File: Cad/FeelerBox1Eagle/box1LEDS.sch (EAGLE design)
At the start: 13 parts

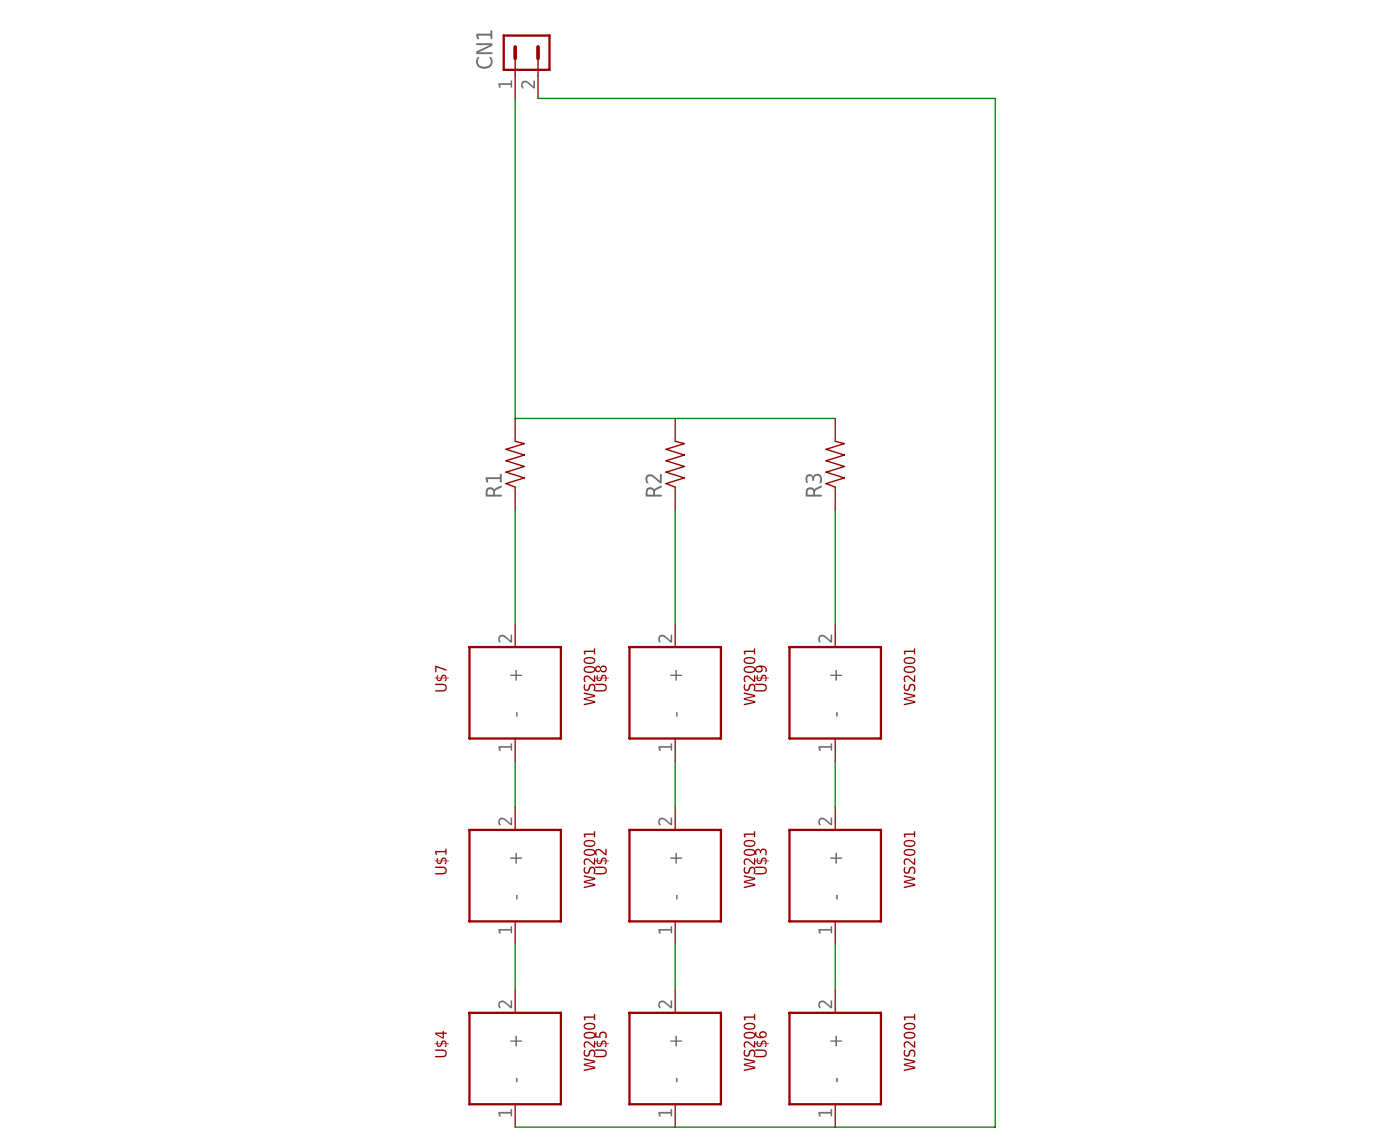
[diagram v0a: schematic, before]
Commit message: updates
bah
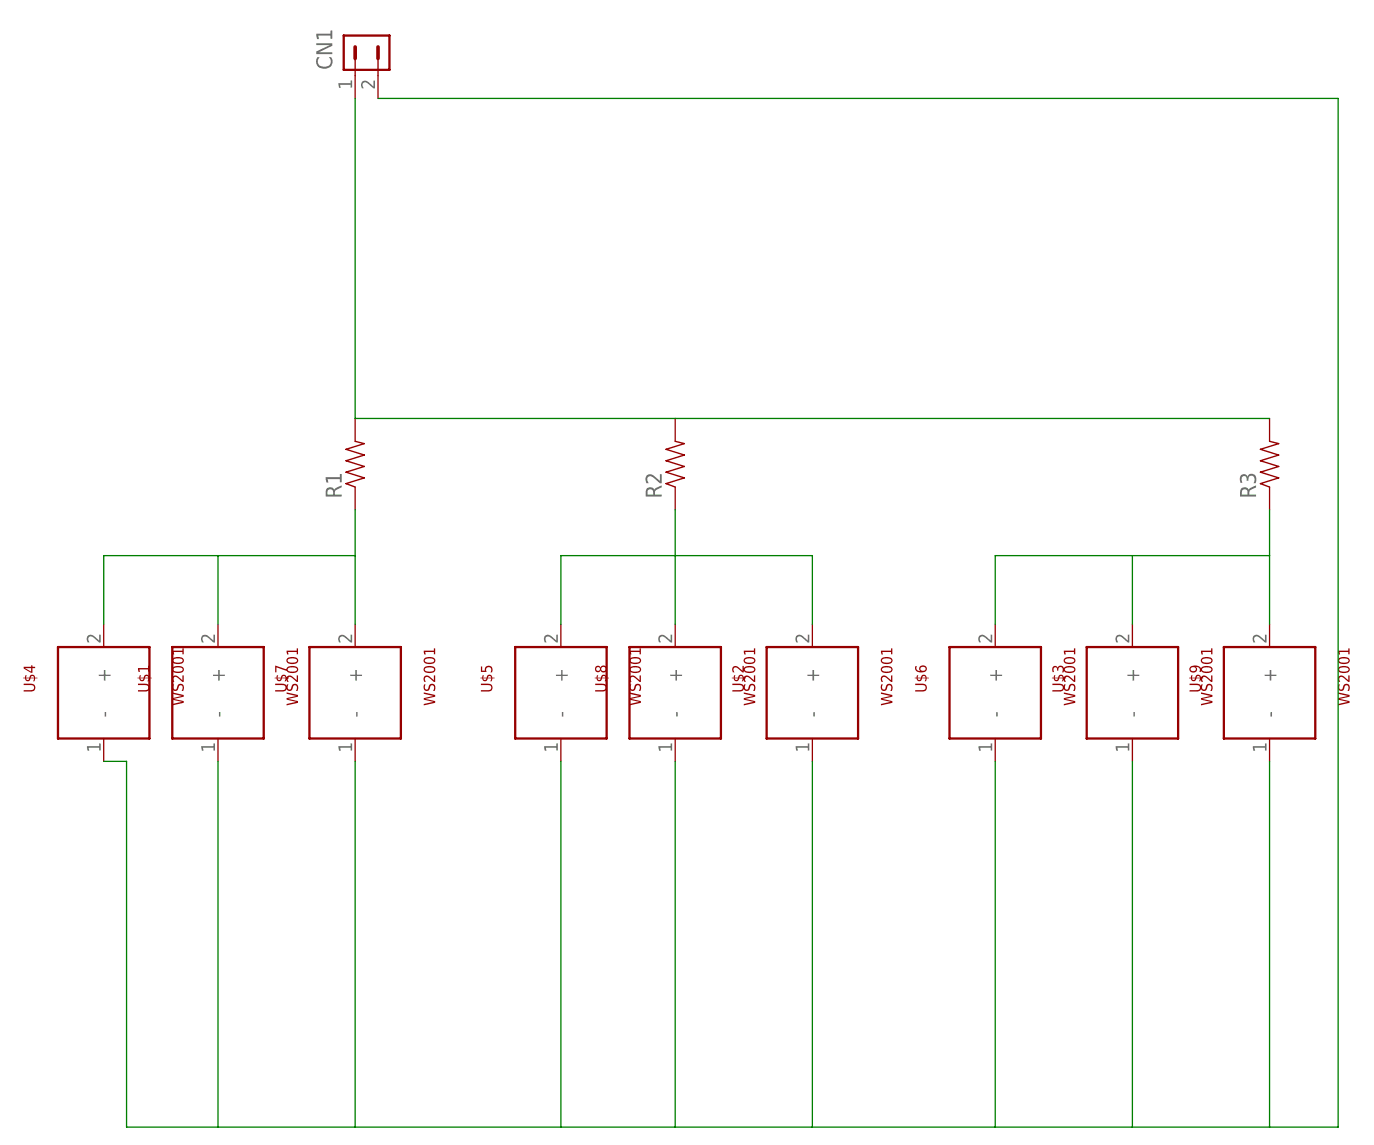
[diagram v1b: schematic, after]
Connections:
- removed net N$20: U$1.+, U$7.-
- removed net N$21: U$2.+, U$8.-
- removed net N$22: U$3.+, U$9.-
- removed net N$23: U$3.-, U$6.+
- removed net N$24: U$2.-, U$5.+
- removed net N$25: U$1.-, U$4.+
- removed net N$4: CN1.2, U$4.-, U$5.-, U$6.-
- new net GND: CN1.2, U$1.-, U$2.-, U$3.-, U$4.-, U$5.-, U$6.-, U$7.-, U$8.-, U$9.-
- net N$1: now also U$3.+, U$6.+
- net N$2: now also U$2.+, U$5.+
- net N$3: now also U$1.+, U$4.+
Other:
- moved on the sheet: CN1, R1, R3, U$1, U$2, U$3, U$4, U$5, U$6, U$7, U$9
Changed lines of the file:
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@@
 </plain>
 <instances>
-<instance part="U$1" gate="G$1" x="-2.54" y="48.26"/>
-<instance part="U$2" gate="G$1" x="15.24" y="48.26"/>
-<instance part="U$3" gate="G$1" x="33.02" y="48.26"/>
-<instance part="U$4" gate="G$1" x="-2.54" y="27.94"/>
-<instance part="U$5" gate="G$1" x="15.24" y="27.94"/>
-<instance part="U$6" gate="G$1" x="33.02" y="27.94"/>
-<instance part="U$7" gate="G$1" x="-2.54" y="68.58"/>
+<instance part="U$1" gate="G$1" x="-35.56" y="68.58"/>
+<instance part="U$2" gate="G$1" x="30.48" y="68.58"/>
+<instance part="U$3" gate="G$1" x="66.04" y="68.58"/>
+<instance part="U$4" gate="G$1" x="-48.26" y="68.58"/>
+<instance part="U$5" gate="G$1" x="2.54" y="68.58"/>
+<instance part="U$6" gate="G$1" x="50.8" y="68.58"/>
+<instance part="U$7" gate="G$1" x="-20.32" y="68.58"/>
 <instance part="U$8" gate="G$1" x="15.24" y="68.58"/>
-<instance part="U$9" gate="G$1" x="33.02" y="68.58"/>
-<instance part="R1" gate="G$1" x="-2.54" y="93.98" rot="R90"/>
+<instance part="U$9" gate="G$1" x="81.28" y="68.58"/>
+<instance part="R1" gate="G$1" x="-20.32" y="93.98" rot="R90"/>
 <instance part="R2" gate="G$1" x="15.24" y="93.98" rot="R90"/>
-<instance part="R3" gate="G$1" x="33.02" y="93.98" rot="R90"/>
-<instance part="CN1" gate="G$1" x="-2.54" y="139.7" rot="R90"/>
+<instance part="R3" gate="G$1" x="81.28" y="93.98" rot="R90"/>
+<instance part="CN1" gate="G$1" x="-20.32" y="139.7" rot="R90"/>
 </instances>
 <busses>
 </busses>
 <nets>
-<net name="N$20" class="0">
-<segment>
-<pinref part="U$1" gate="G$1" pin="+"/>
-<pinref part="U$7" gate="G$1" pin="-"/>
-<wire x1="-2.54" y1="55.88" x2="-2.54" y2="60.96" width="0.1524" layer="91"/>
-</segment>
-</net>
-<net name="N$21" class="0">
-<segment>
-<pinref part="U$2" gate="G$1" pin="+"/>
-<pinref part="U$8" gate="G$1" pin="-"/>
-<wire x1="15.24" y1="55.88" x2="15.24" y2="60.96" width="0.1524" layer="91"/>
-</segment>
-</net>
-<net name="N$22" class="0">
-<segment>
-<pinref part="U$3" gate="G$1" pin="+"/>
-<pinref part="U$9" gate="G$1" pin="-"/>
-<wire x1="33.02" y1="55.88" x2="33.02" y2="60.96" width="0.1524" layer="91"/>
-</segment>
-</net>
-<net name="N$23" class="0">
-<segment>
-<pinref part="U$6" gate="G$1" pin="+"/>
-<pinref part="U$3" gate="G$1" pin="-"/>
-<wire x1="33.02" y1="35.56" x2="33.02" y2="40.64" width="0.1524" layer="91"/>
-</segment>
-</net>
-<net name="N$24" class="0">
-<segment>
-<pinref part="U$5" gate="G$1" pin="+"/>
-<pinref part="U$2" gate="G$1" pin="-"/>
-<wire x1="15.24" y1="35.56" x2="15.24" y2="40.64" width="0.1524" layer="91"/>
-</segment>
-</net>
-<net name="N$25" class="0">
-<segment>
-<pinref part="U$4" gate="G$1" pin="+"/>
-<pinref part="U$1" gate="G$1" pin="-"/>
-<wire x1="-2.54" y1="35.56" x2="-2.54" y2="40.64" width="0.1524" layer="91"/>
-</segment>
-</net>
 <net name="N$1" class="0">
 <segment>
 <pinref part="U$9" gate="G$1" pin="+"/>
 <pinref part="R3" gate="G$1" pin="1"/>
-<wire x1="33.02" y1="76.2" x2="33.02" y2="88.9" width="0.1524" layer="91"/>
+<wire x1="81.28" y1="76.2" x2="81.28" y2="83.82" width="0.1524" layer="91"/>
+<pinref part="U$6" gate="G$1" pin="+"/>
+<wire x1="50.8" y1="76.2" x2="50.8" y2="83.82" width="0.1524" layer="91"/>
+<wire x1="50.8" y1="83.82" x2="66.04" y2="83.82" width="0.1524" layer="91"/>
+<wire x1="66.04" y1="83.82" x2="81.28" y2="83.82" width="0.1524" layer="91"/>
+<wire x1="81.28" y1="83.82" x2="81.28" y2="88.9" width="0.1524" layer="91"/>
+<pinref part="U$3" gate="G$1" pin="+"/>
+<wire x1="66.04" y1="76.2" x2="66.04" y2="83.82" width="0.1524" layer="91"/>
 </segment>
 </net>
@@
 <pinref part="U$8" gate="G$1" pin="+"/>
 <pinref part="R2" gate="G$1" pin="1"/>
-<wire x1="15.24" y1="76.2" x2="15.24" y2="88.9" width="0.1524" layer="91"/>
+<wire x1="15.24" y1="76.2" x2="15.24" y2="83.82" width="0.1524" layer="91"/>
+<pinref part="U$2" gate="G$1" pin="+"/>
+<wire x1="15.24" y1="83.82" x2="15.24" y2="88.9" width="0.1524" layer="91"/>
+<wire x1="15.24" y1="83.82" x2="30.48" y2="83.82" width="0.1524" layer="91"/>
+<wire x1="30.48" y1="83.82" x2="30.48" y2="76.2" width="0.1524" layer="91"/>
+<pinref part="U$5" gate="G$1" pin="+"/>
+<wire x1="15.24" y1="83.82" x2="2.54" y2="83.82" width="0.1524" layer="91"/>
+<wire x1="2.54" y1="83.82" x2="2.54" y2="76.2" width="0.1524" layer="91"/>
 </segment>
 </net>
@@
 <pinref part="U$7" gate="G$1" pin="+"/>
 <pinref part="R1" gate="G$1" pin="1"/>
-<wire x1="-2.54" y1="76.2" x2="-2.54" y2="88.9" width="0.1524" layer="91"/>
+<wire x1="-20.32" y1="76.2" x2="-20.32" y2="83.82" width="0.1524" layer="91"/>
+<wire x1="-20.32" y1="83.82" x2="-20.32" y2="88.9" width="0.1524" layer="91"/>
+<wire x1="-20.32" y1="83.82" x2="-35.56" y2="83.82" width="0.1524" layer="91"/>
+<pinref part="U$4" gate="G$1" pin="+"/>
+<wire x1="-35.56" y1="83.82" x2="-48.26" y2="83.82" width="0.1524" layer="91"/>
+<wire x1="-48.26" y1="83.82" x2="-48.26" y2="76.2" width="0.1524" layer="91"/>
+<pinref part="U$1" gate="G$1" pin="+"/>
+<wire x1="-35.56" y1="76.2" x2="-35.56" y2="83.82" width="0.1524" layer="91"/>
 </segment>
 </net>
@@
 <pinref part="R3" gate="G$1" pin="2"/>
 <pinref part="R2" gate="G$1" pin="2"/>
-<wire x1="33.02" y1="99.06" x2="15.24" y2="99.06" width="0.1524" layer="91"/>
+<wire x1="81.28" y1="99.06" x2="15.24" y2="99.06" width="0.1524" layer="91"/>
 <pinref part="R1" gate="G$1" pin="2"/>
-<wire x1="-2.54" y1="99.06" x2="15.24" y2="99.06" width="0.1524" layer="91"/>
-<wire x1="-2.54" y1="99.06" x2="-2.54" y2="134.62" width="0.1524" layer="91"/>
+<wire x1="-20.32" y1="99.06" x2="15.24" y2="99.06" width="0.1524" layer="91"/>
+<wire x1="-20.32" y1="99.06" x2="-20.32" y2="134.62" width="0.1524" layer="91"/>
 <pinref part="CN1" gate="G$1" pin="1"/>
 </segment>
 </net>
-<net name="N$4" class="0">
+<net name="GND" class="0">
 <segment>
 <pinref part="CN1" gate="G$1" pin="2"/>
-<wire x1="0" y1="134.62" x2="50.8" y2="134.62" width="0.1524" layer="91"/>
-<wire x1="50.8" y1="134.62" x2="50.8" y2="20.32" width="0.1524" layer="91"/>
+<wire x1="-17.78" y1="134.62" x2="88.9" y2="134.62" width="0.1524" layer="91"/>
+<wire x1="88.9" y1="134.62" x2="88.9" y2="20.32" width="0.1524" layer="91"/>
+<pinref part="U$4" gate="G$1" pin="-"/>
+<wire x1="-48.26" y1="60.96" x2="-45.72" y2="60.96" width="0.1524" layer="91"/>
+<wire x1="-45.72" y1="60.96" x2="-45.72" y2="20.32" width="0.1524" layer="91"/>
+<wire x1="-45.72" y1="20.32" x2="-35.56" y2="20.32" width="0.1524" layer="91"/>
+<pinref part="U$1" gate="G$1" pin="-"/>
+<wire x1="-35.56" y1="20.32" x2="-20.32" y2="20.32" width="0.1524" layer="91"/>
+<wire x1="-20.32" y1="20.32" x2="2.54" y2="20.32" width="0.1524" layer="91"/>
+<wire x1="2.54" y1="20.32" x2="15.24" y2="20.32" width="0.1524" layer="91"/>
+<wire x1="15.24" y1="20.32" x2="30.48" y2="20.32" width="0.1524" layer="91"/>
+<wire x1="30.48" y1="20.32" x2="50.8" y2="20.32" width="0.1524" layer="91"/>
+<wire x1="50.8" y1="20.32" x2="66.04" y2="20.32" width="0.1524" layer="91"/>
+<wire x1="66.04" y1="20.32" x2="81.28" y2="20.32" width="0.1524" layer="91"/>
+<wire x1="81.28" y1="20.32" x2="88.9" y2="20.32" width="0.1524" layer="91"/>
+<wire x1="-35.56" y1="60.96" x2="-35.56" y2="20.32" width="0.1524" layer="91"/>
+<pinref part="U$7" gate="G$1" pin="-"/>
+<wire x1="-20.32" y1="60.96" x2="-20.32" y2="20.32" width="0.1524" layer="91"/>
+<pinref part="U$5" gate="G$1" pin="-"/>
+<wire x1="2.54" y1="60.96" x2="2.54" y2="20.32" width="0.1524" layer="91"/>
+<pinref part="U$8" gate="G$1" pin="-"/>
+<wire x1="15.24" y1="60.96" x2="15.24" y2="20.32" width="0.1524" layer="91"/>
+<pinref part="U$2" gate="G$1" pin="-"/>
+<wire x1="30.48" y1="60.96" x2="30.48" y2="20.32" width="0.1524" layer="91"/>
+<pinref part="U$3" gate="G$1" pin="-"/>
+<wire x1="66.04" y1="60.96" x2="66.04" y2="20.32" width="0.1524" layer="91"/>
+<pinref part="U$9" gate="G$1" pin="-"/>
+<wire x1="81.28" y1="60.96" x2="81.28" y2="20.32" width="0.1524" layer="91"/>
 <pinref part="U$6" gate="G$1" pin="-"/>
-<wire x1="50.8" y1="20.32" x2="33.02" y2="20.32" width="0.1524" layer="91"/>
-<pinref part="U$5" gate="G$1" pin="-"/>
-<wire x1="33.02" y1="20.32" x2="15.24" y2="20.32" width="0.1524" layer="91"/>
-<pinref part="U$4" gate="G$1" pin="-"/>
-<wire x1="15.24" y1="20.32" x2="-2.54" y2="20.32" width="0.1524" layer="91"/>
+<wire x1="50.8" y1="60.96" x2="50.8" y2="20.32" width="0.1524" layer="91"/>
 </segment>
 </net>
